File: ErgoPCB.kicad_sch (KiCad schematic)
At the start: 18 parts, among them J1 Conn_01x04_MountingPin, U1 SRV05-4, U2 XC6206PxxxMR, U3 STM32F072CBT6

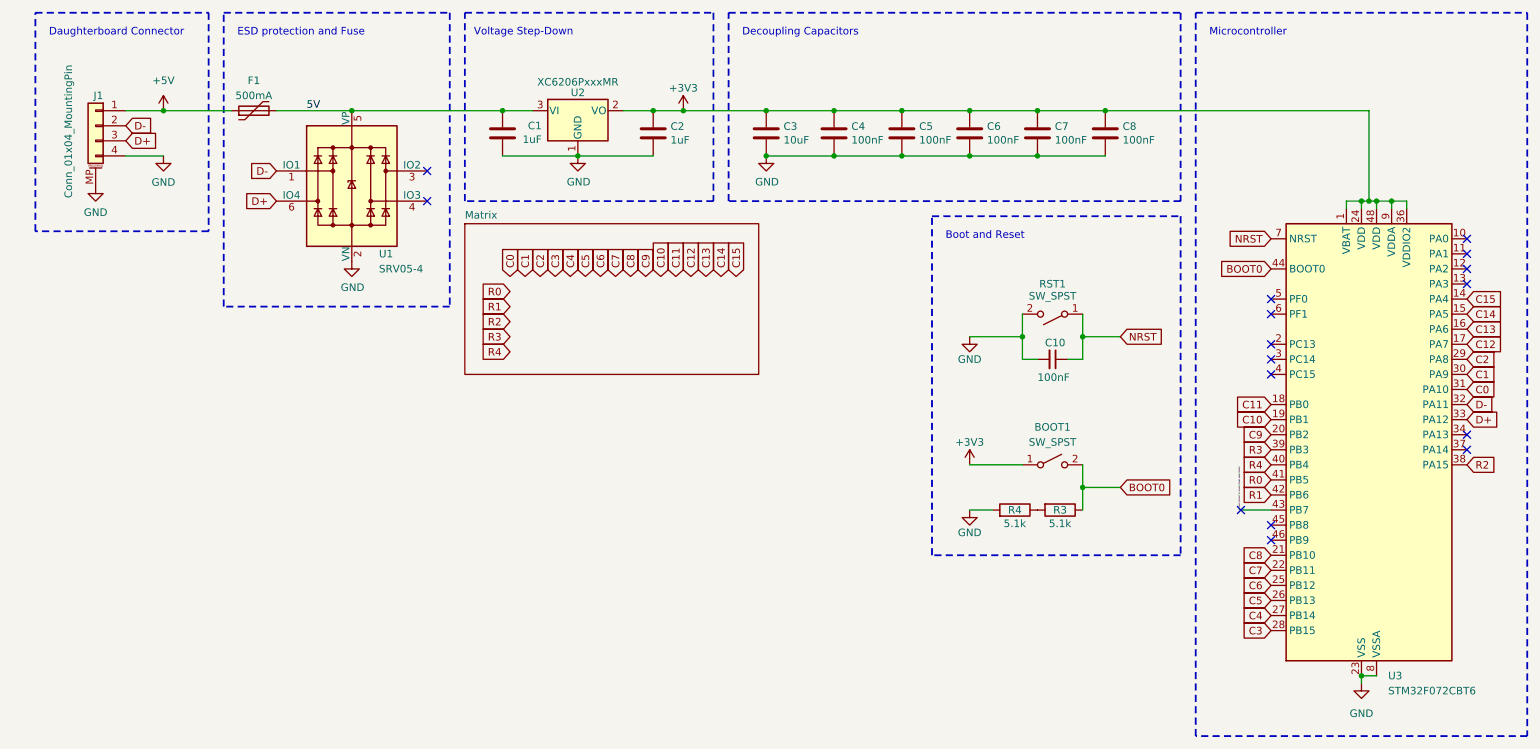
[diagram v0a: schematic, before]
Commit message: Small changes
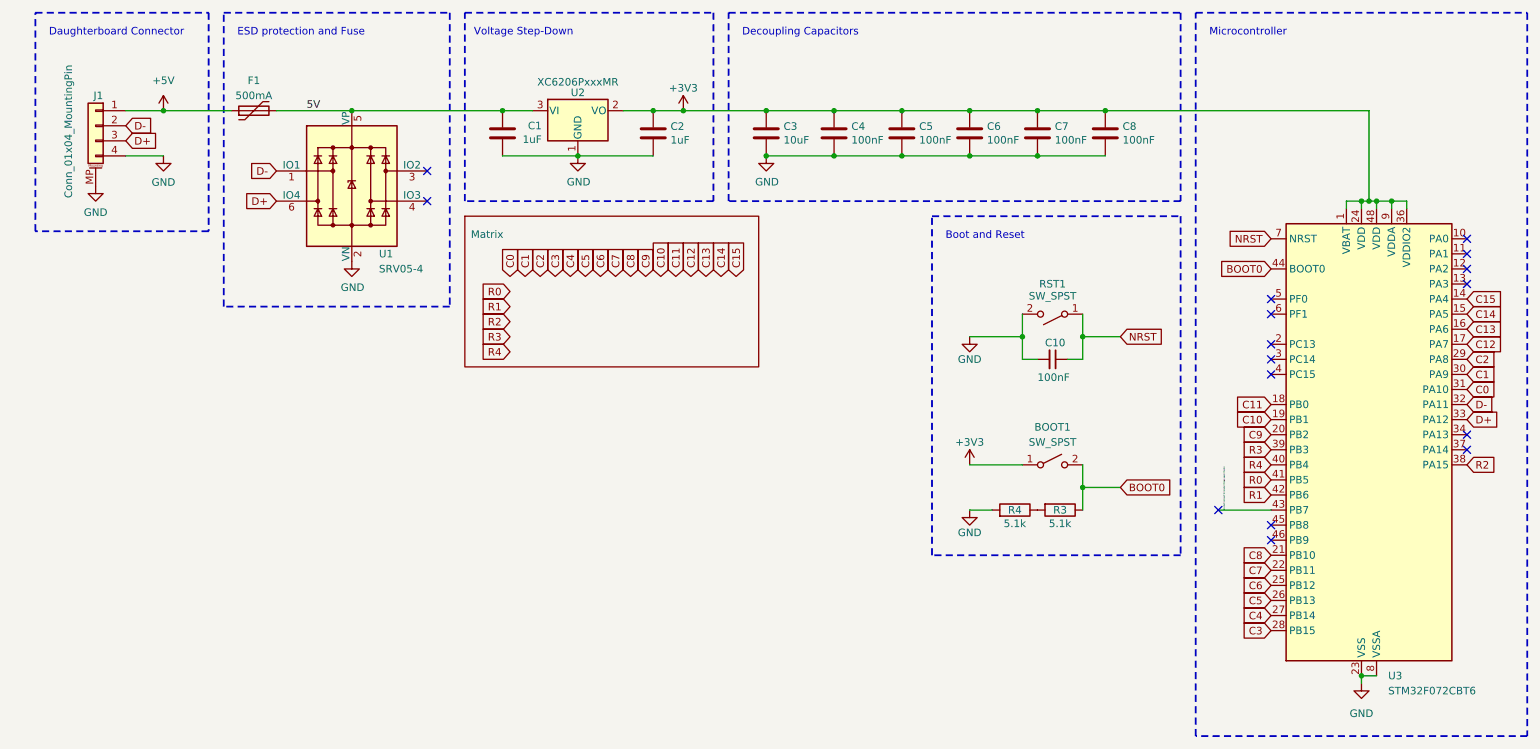
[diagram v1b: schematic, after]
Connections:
- net pls dont connect to randon things again thanks renamed     pls dont connect to randon things again thanks
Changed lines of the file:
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@@
 	)
 	(no_connect
-		(at 226.06 111.76)
+		(at 222.25 111.76)
 	)
 	(no_connect
@@
 	(wire
 		(pts
-			(xy 248.92 59.69) (xy 248.92 60.96)
+			(xy 222.25 111.76) (xy 231.14 111.76)
 		)
 		(stroke
@@
 	(wire
 		(pts
-			(xy 199.39 107.95) (xy 199.39 111.76)
+			(xy 248.92 59.69) (xy 248.92 60.96)
 		)
 		(stroke
@@
 	(wire
 		(pts
-			(xy 189.23 86.36) (xy 189.23 82.55)
+			(xy 199.39 107.95) (xy 199.39 111.76)
 		)
 		(stroke
@@
 	(wire
 		(pts
-			(xy 38.1 52.07) (xy 44.45 52.07)
+			(xy 189.23 86.36) (xy 189.23 82.55)
 		)
 		(stroke
@@
 	(wire
 		(pts
-			(xy 251.46 59.69) (xy 251.46 60.96)
+			(xy 38.1 52.07) (xy 44.45 52.07)
 		)
 		(stroke
@@
 	(wire
 		(pts
-			(xy 191.77 44.45) (xy 203.2 44.45)
+			(xy 251.46 59.69) (xy 251.46 60.96)
 		)
 		(stroke
@@
 	(wire
 		(pts
-			(xy 226.06 111.76) (xy 231.14 111.76)
+			(xy 191.77 44.45) (xy 203.2 44.45)
 		)
 		(stroke
@@
 		)
 	)
-	(label "pls dont connect to randon things again thanks"
-		(at 226.06 111.76 90)
+	(label "    pls dont connect to randon things again thanks"
+		(at 223.52 111.76 90)
 		(effects
 			(font
@@
 	)
 	(sheet
-		(at 95.25 63.5)
+		(at 95.25 62.23)
 		(size 49.53 25.4)
-		(fields_autoplaced yes)
 		(stroke
 			(width 0.15)
@@
 		)
 		(property "Sheetname" "Matrix"
-			(at 95.25 62.7884 0)
+			(at 96.266 66.04 0)
 			(effects
 				(font
@@
 		)
 		(property "Sheetfile" "Matrix.kicad_sch"
-			(at 95.25 89.4846 0)
+			(at 95.25 88.2146 0)
 			(effects
 				(font

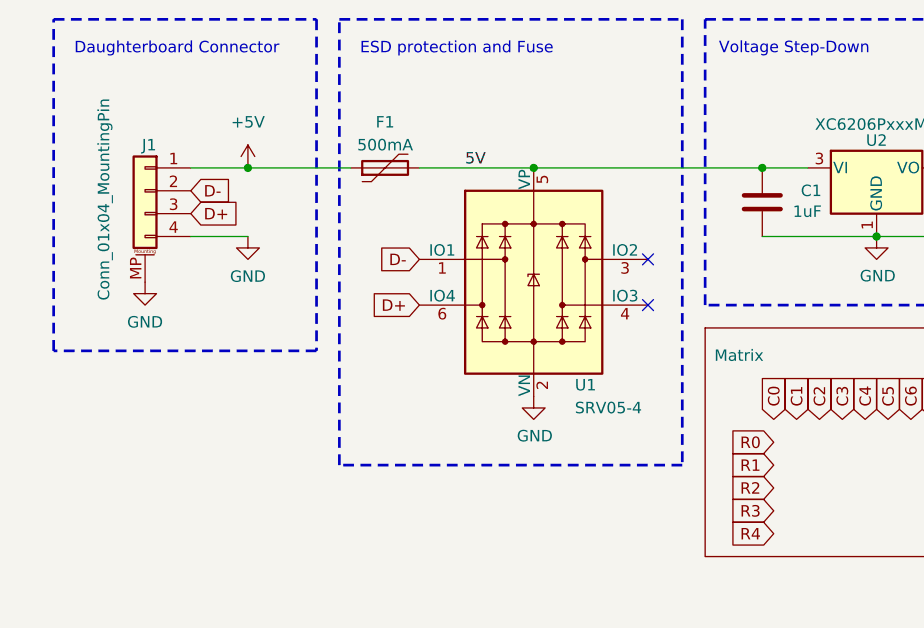
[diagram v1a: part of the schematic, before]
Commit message: Small fixes
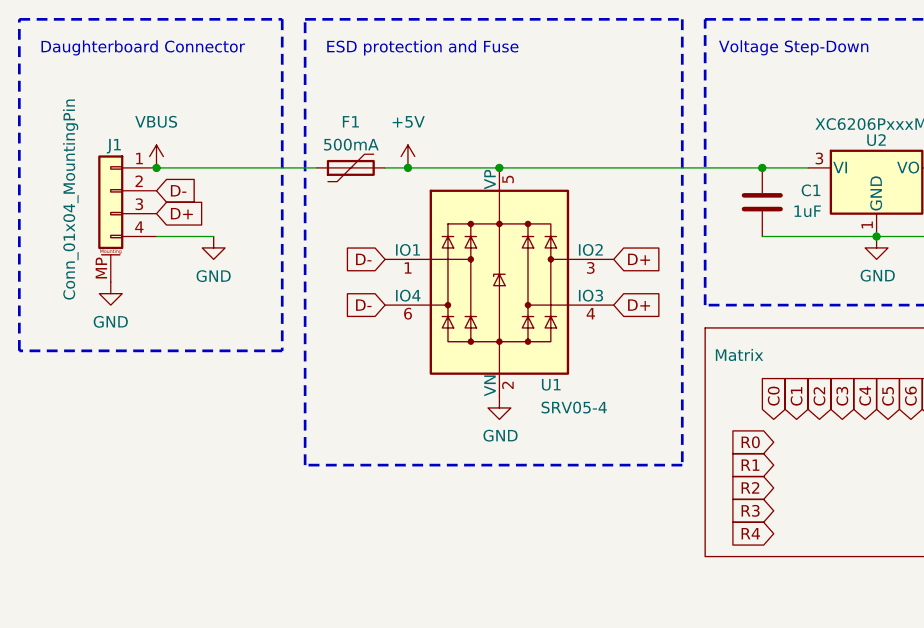
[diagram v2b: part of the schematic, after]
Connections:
- net 5V is gone; now on net +5V: C1.1, F1.2, U1.5 (VP), U2.3 (VI)
- net +5V: no longer F1.1, J1.1 (Pin_1)
- net D+: now also U1.3 (IO2), U1.4 (IO3); no longer U1.6 (IO4)
- net D-: now also U1.6 (IO4)
- new net VBUS: F1.1, J1.1 (Pin_1)
- no-connect marks 16 -> 14
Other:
- moved on the sheet: F1, J1, U1
